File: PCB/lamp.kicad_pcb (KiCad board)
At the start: 2 copper layers, 23.5 x 25.5 mm, 3 parts, among them Q1 NMOS, U1 XIAO ESP32C3

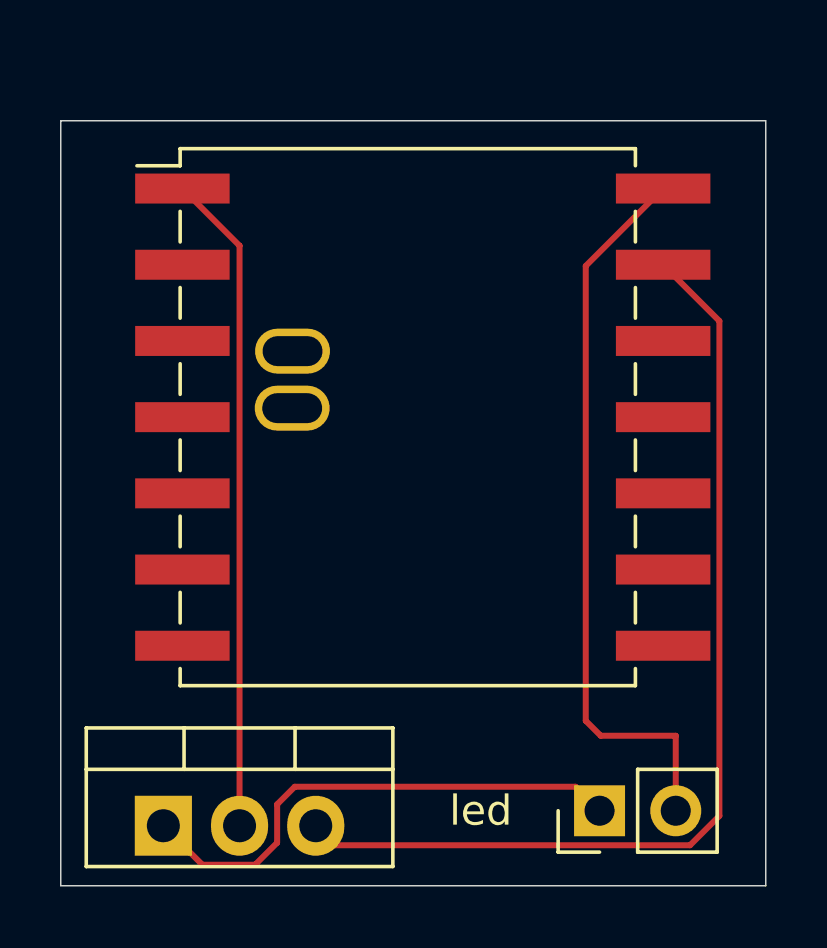
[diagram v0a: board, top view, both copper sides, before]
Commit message: Add files via upload
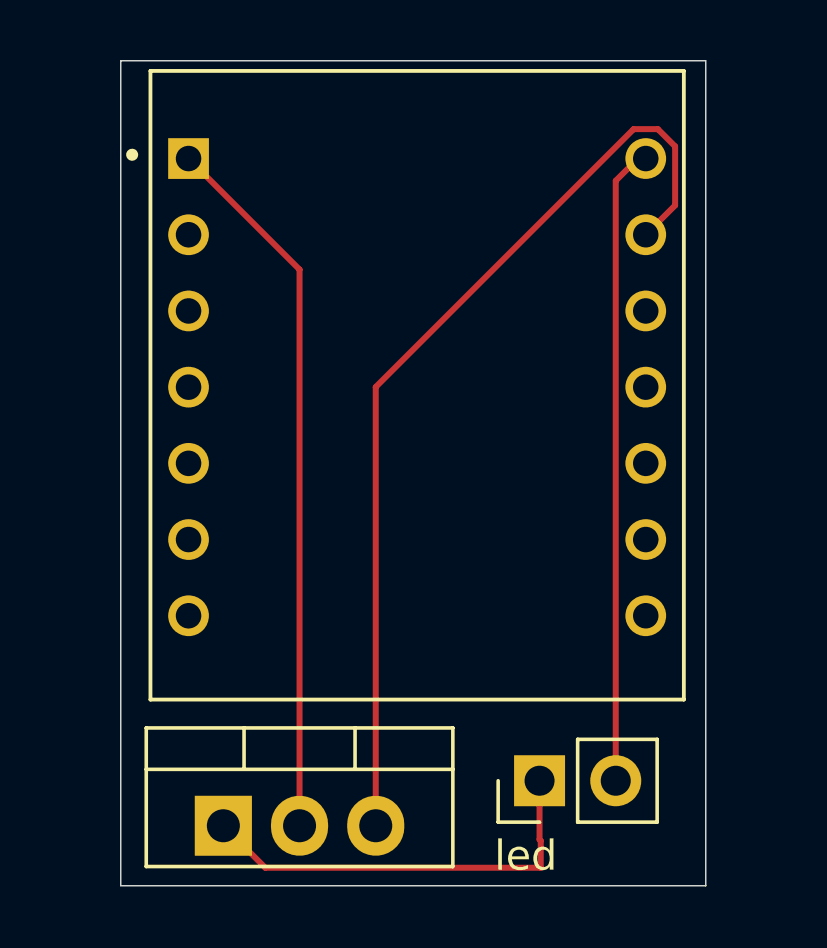
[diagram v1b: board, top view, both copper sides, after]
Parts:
- U1: value XIAO ESP32C3 -> XIAO_ESP32C3
- moved U1 2.97 mm to (118.4, 83.8)
- moved led 2.24 mm to (122.5, 97.0)
- moved Q1 2.00 mm to (111.9, 98.5)
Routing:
- net Net-(Q1-D): track 17.2 -> 14.1 mm
- net Net-(U1-VUSB): track 24.5 -> 21.7 mm
- net Net-(Q1-G): track 22.0 -> 23.8 mm
- net Net-(Q1-S): track 33.3 -> 31.8 mm
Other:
- board size 23.5 x 25.5 mm -> 19.5 x 27.5 mm
